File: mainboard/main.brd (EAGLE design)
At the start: 53.4 x 45.7 mm, 4 parts, among them J1 RJHSE-3380, J2 RJHSE-3380, J3 RJHSE-3380

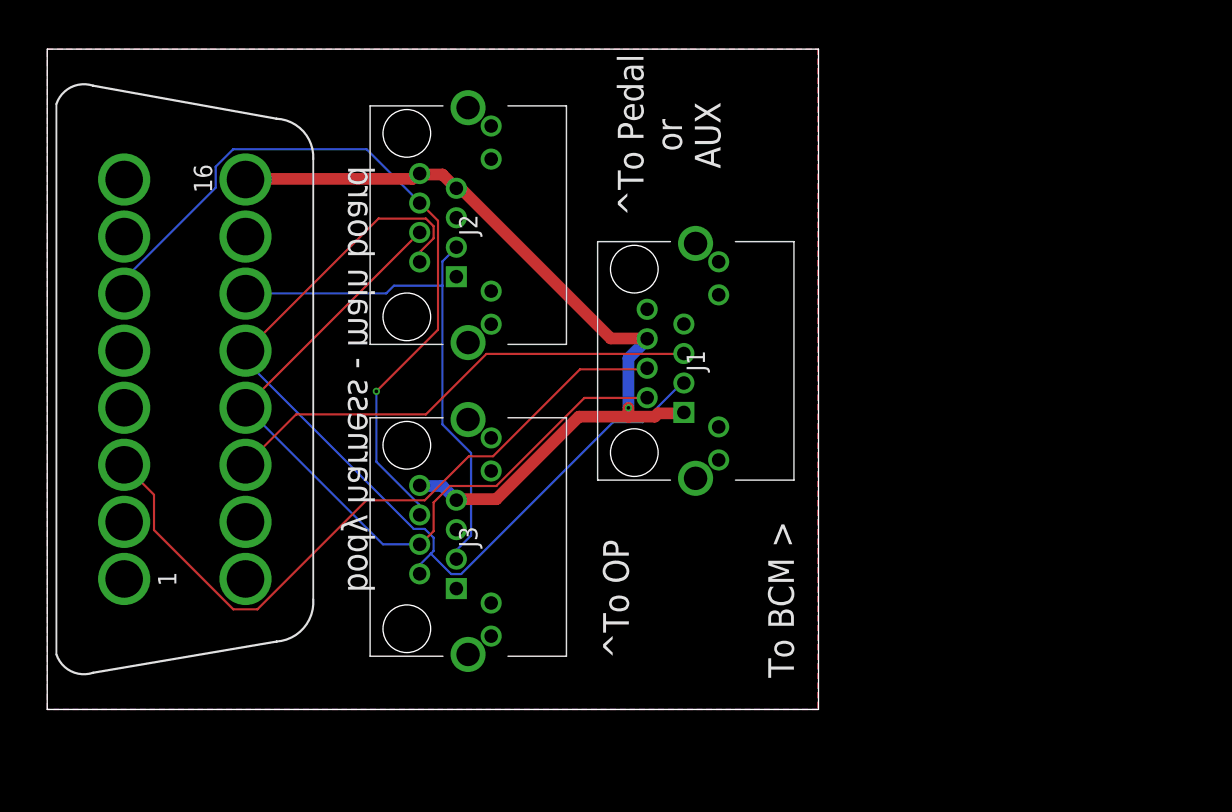
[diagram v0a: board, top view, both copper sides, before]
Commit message: main v2
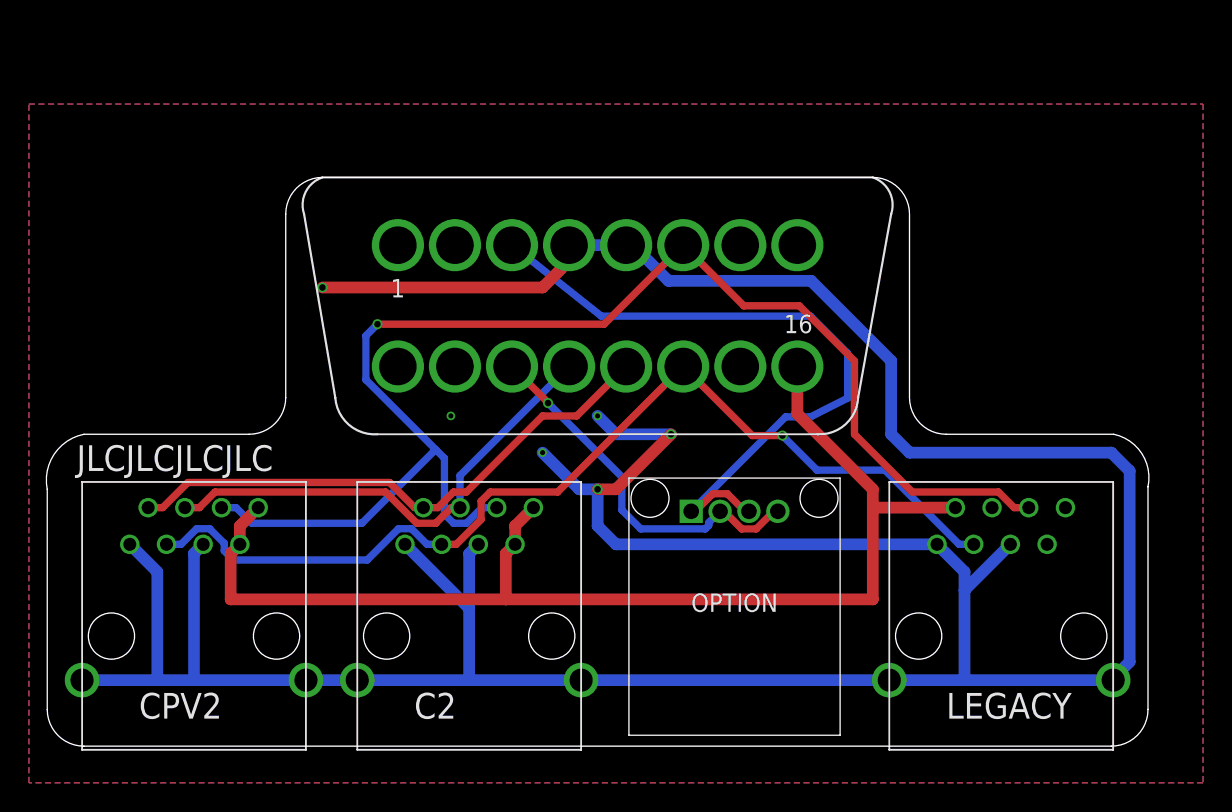
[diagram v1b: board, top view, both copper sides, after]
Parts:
- removed J1, J2, J3: RJHSE-3380, RJHSE-3380:RJHSE3384
- added C2, CPV2, LEGACY: RA-RJ45RA, comma.ai:RA-RJ45
- added OPTION: 34793-0041, 34793-0041:347930041
- moved PANDA 29.0 mm to (38.1, 27.9), turned to 180 degrees
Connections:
- net CAN0_H: now also C2.6, CPV2.6, LEGACY.6; no longer J2.6, J3.6
- net CAN0_L: now also C2.3, CPV2.3, LEGACY.3; no longer J2.3, J3.3
- net CAN1_H: now also OPTION.1, OPTION.3; no longer J1.4
- net CAN1_L: now also OPTION.2, OPTION.4; no longer J1.5
- net CAN2_H: now also C2.4, CPV2.4; no longer J1.2, J2.4, J3.4
- net CAN2_L: now also C2.2, CPV2.2; no longer J1.3, J2.2, J3.2
- net GND: now also C2.1, C2.5, C2.P$1, C2.P$2, CPV2.1, CPV2.5, CPV2.P$1, CPV2.P$2, LEGACY.1, LEGACY.5, LEGACY.P$1, LEGACY.P$2; no longer J1.7, J1.8, J2.1, J2.5, J3.1, J3.5
- net VIN: now also C2.7, C2.8, CPV2.7, CPV2.8, LEGACY.2; no longer J1.1, J1.6, J2.7, J2.8, J3.7, J3.8
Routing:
- net GND: track 0.00 -> 247.7 mm, vias 0 -> 6
- net CAN0_H: track 52.7 -> 95.3 mm
- net CAN0_L: track 37.1 -> 69.8 mm, vias 0 -> 1
- net CAN2_L: track 65.2 -> 38.6 mm
- net VIN: track 59.9 -> 82.7 mm, vias 1 -> 0
- net CAN2_H: track 54.2 -> 33.7 mm
- net CAN1_L: track 33.5 -> 26.0 mm, vias 0 -> 1
- net CAN1_H: track 48.7 -> 48.0 mm
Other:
- board size 53.4 x 45.7 mm -> 76.3 x 39.4 mm
- board text added: "JLCJLCJLCJLC"
- board text added: "body harness - main"
- board text added: "csouers 8/18/2020"
- board text added: "github.com/csouers"
- board text removed: "To BCM >"
- board text removed: "^To OP"
- board text removed: "^To Pedal or AUX"
- board text removed: "body harness - main board"
- board text removed: "csouers 7/1/2020"
- board text removed: "github.com/csouers/bodyharness"
